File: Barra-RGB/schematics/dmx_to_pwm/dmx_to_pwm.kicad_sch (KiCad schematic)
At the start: 36 parts, among them IC1 LM1085IT-12_NOPB, J4 PJ-031D, SW1 SW_SPDT, SW2 SW_SPDT, SW3 SW_SPDT, U1 SN75176AP, U2 6N137, U3 6N137, U4 SN75176AP

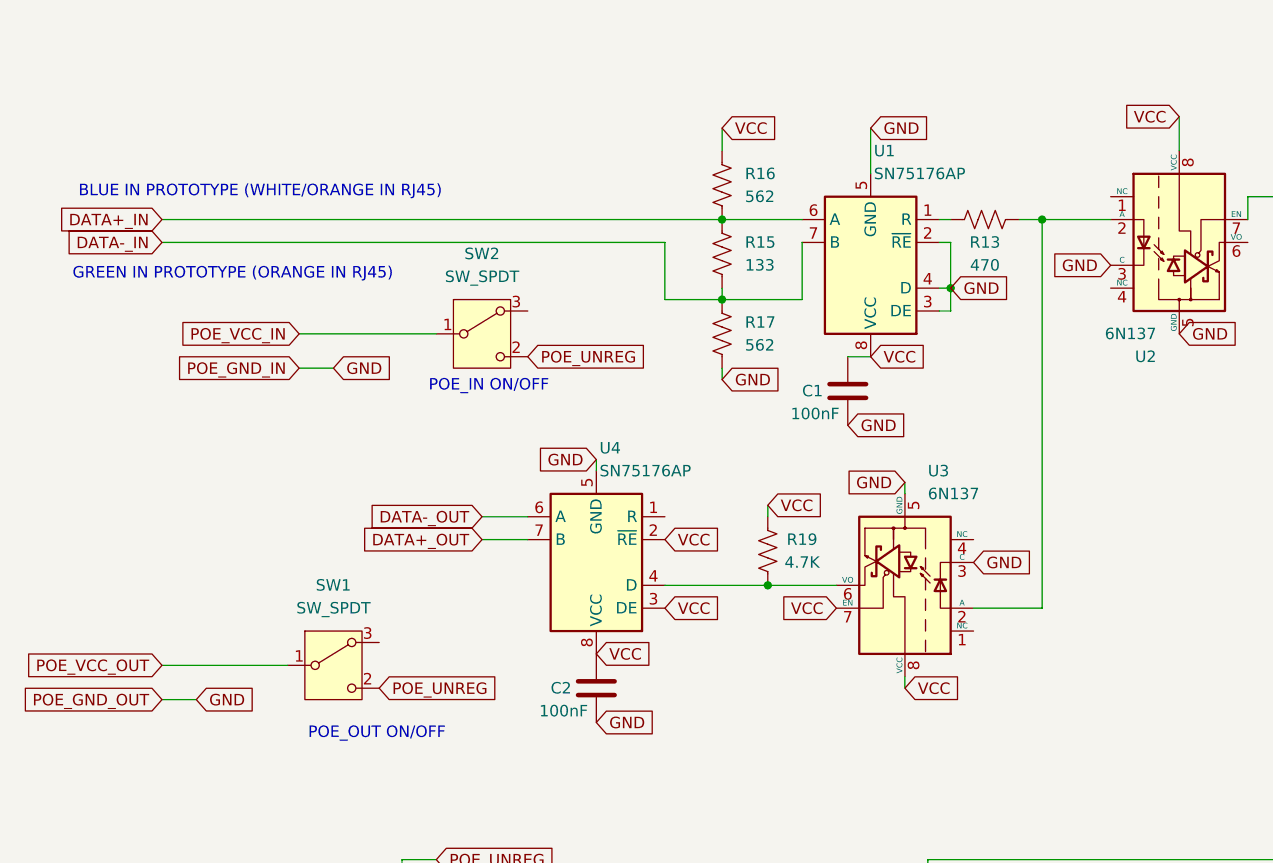
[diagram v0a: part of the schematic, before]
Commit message: debugging
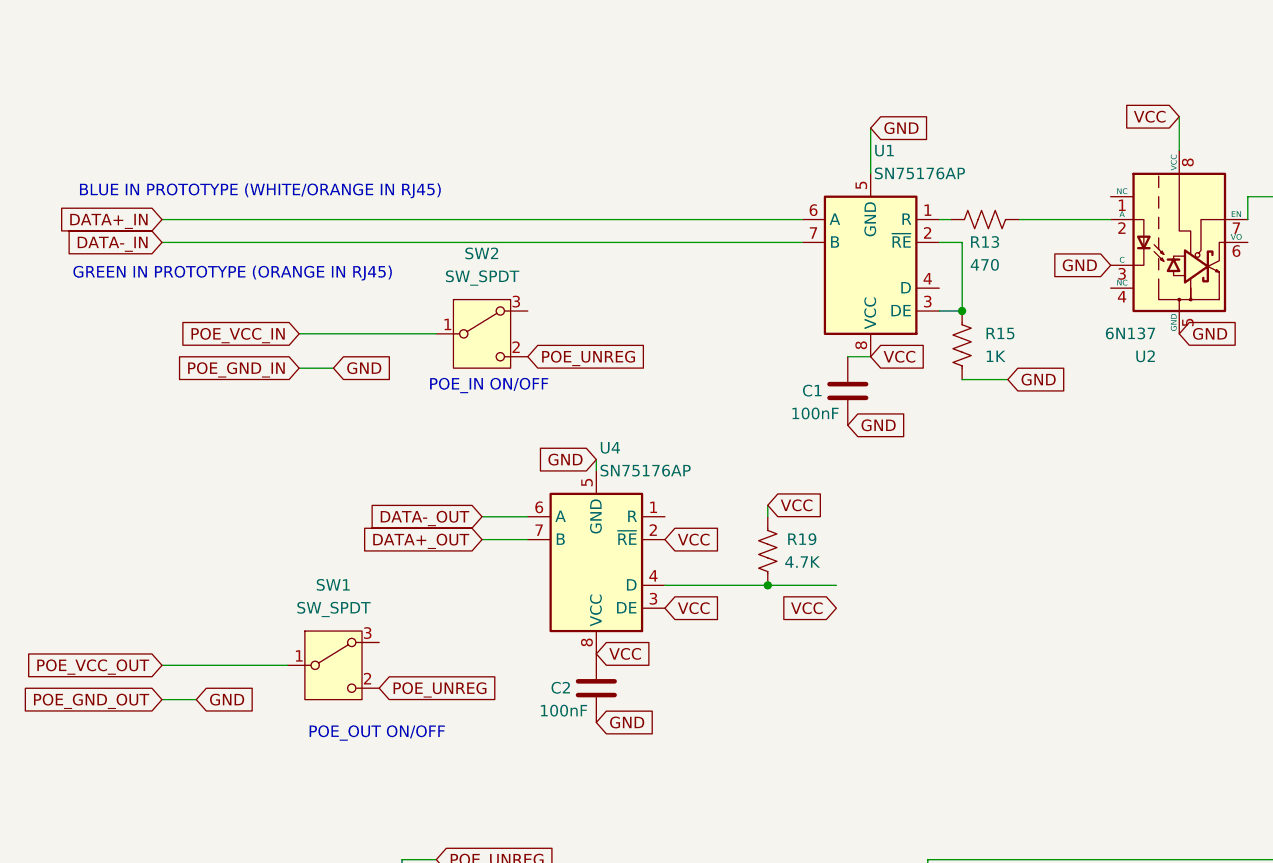
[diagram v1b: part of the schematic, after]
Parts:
- removed R16, R17: 562, Resistor_THT:R_Axial_DIN0204_L3.6mm_D1.6mm_P7.62mm_Horizontal, symbol Device:R_US
- removed U3: 6N137, Package_DIP:DIP-8_W7.62mm, symbol Isolator:6N137
- R15: value 133 -> 1K; footprint Resistor_THT:R_Axial_DIN0204_L3.6mm_D1.6mm_P7.62mm_Horizontal -> (none)
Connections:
- net DATA+_IN: no longer R15.1
- net DATA-_IN: no longer R15.2
- net DRV1-: now also R15.2; no longer U1.2 (~{RE}), U1.3 (DE), U1.4 (D)
- new net: R15.1, U1.2 (~{RE}), U1.3 (DE)
